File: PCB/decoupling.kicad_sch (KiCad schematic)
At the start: 9 parts

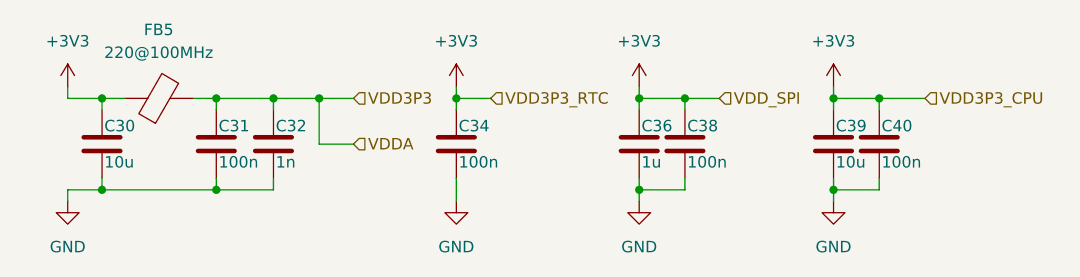
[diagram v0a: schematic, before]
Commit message: big things are happening
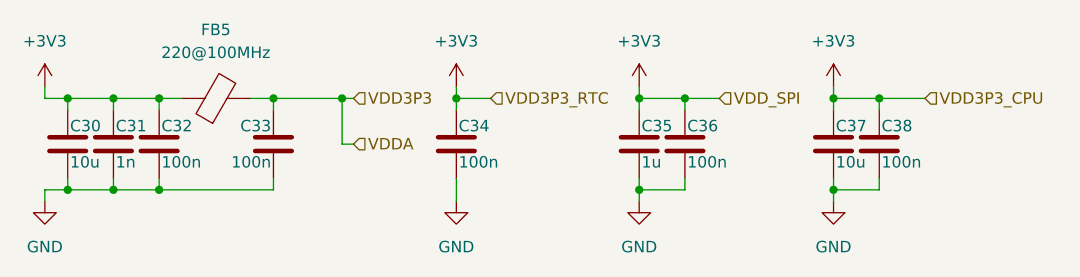
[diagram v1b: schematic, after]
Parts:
- added C32: 100n, Capacitor_SMD:C_0402_1005Metric, symbol Device:C
- FB5: footprint (none) -> Inductor_SMD:L_0805_2012Metric
- renumbered C32 to C31, C31 to C33, C36 to C35, C38 to C36, C39 to C37, C40 to C38
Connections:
- net +3V3: now also C31.1, C32.1
- net GND: now also C32.2
- net VDD3P3: no longer C31.1
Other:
- moved on the sheet: C30, C31, C33, FB5
